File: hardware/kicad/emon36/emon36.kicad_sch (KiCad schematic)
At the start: 80 parts, among them J1 Barrel_Jack, J37 USB_B_Micro, J4 Barrel_Jack, SW1 SW_MEC_5E, SW2 SW_MEC_5E, SW3 SW_MEC_5E, SW4 SW_MEC_5E, SW5 RotaryEncoder, U1 ESP32-C3-WROOM-02-N4, U3 16.384MHz, U8 TPS5403

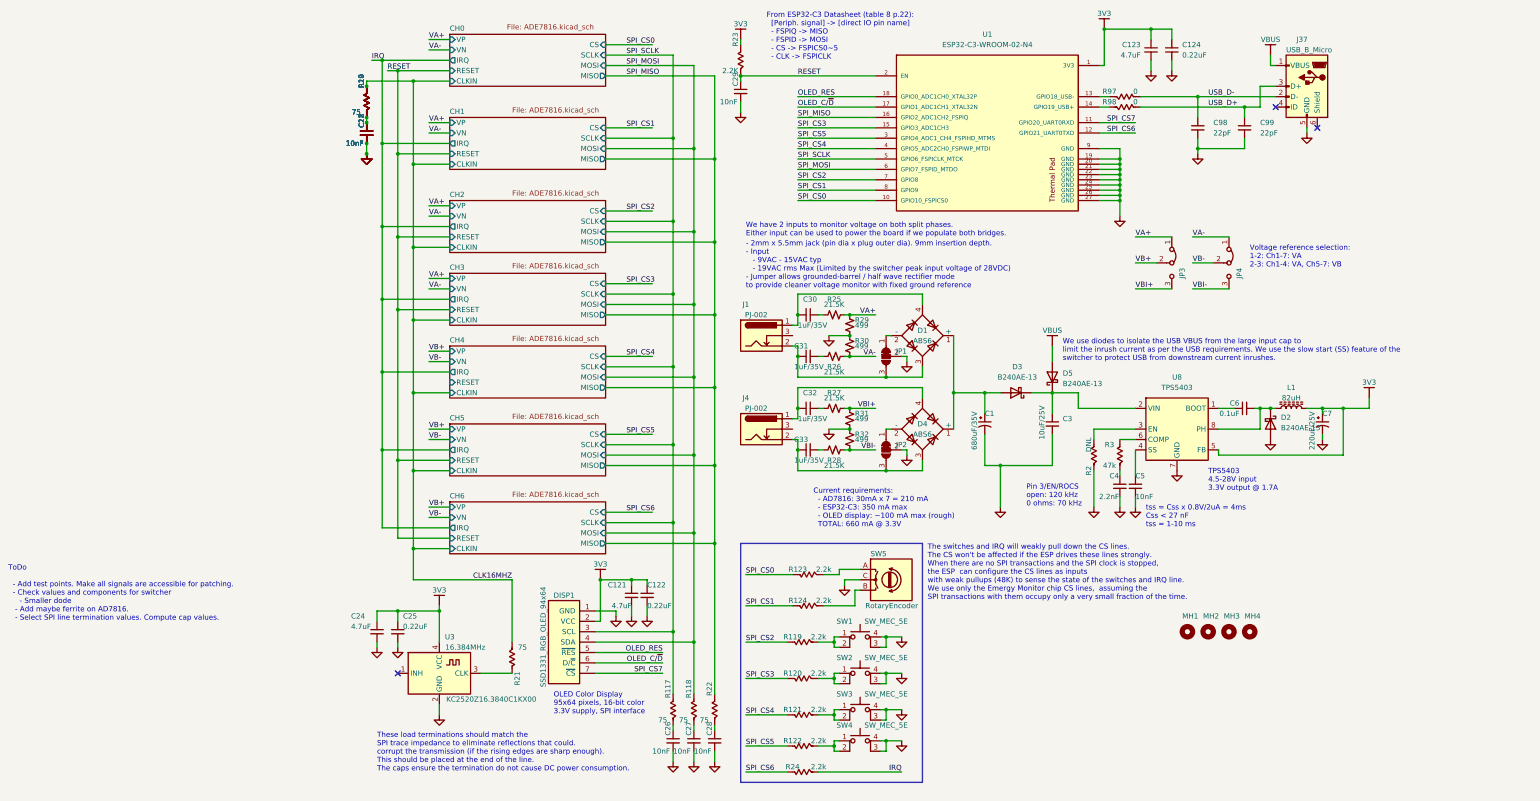
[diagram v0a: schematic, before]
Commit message: Finished schematics, layout and routing. Ready for verification.
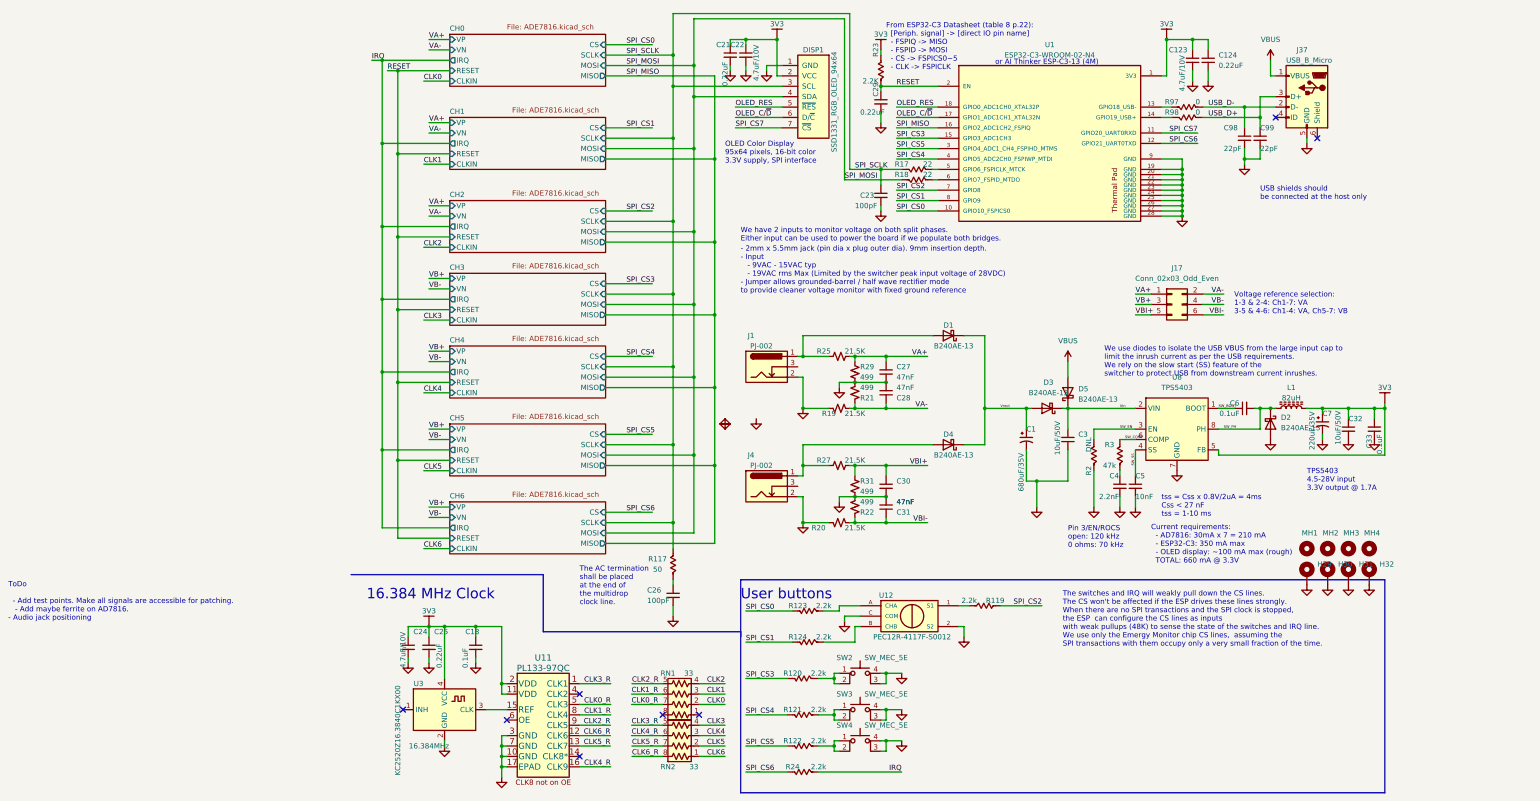
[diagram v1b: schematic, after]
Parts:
- removed C121: 4.7uF, Capacitor_SMD:C_0603_1608Metric, symbol Device:C_Small
- removed C122: 0.22uF, Capacitor_SMD:C_0603_1608Metric, symbol Device:C_Small
- removed D1, D4: ABS6, Diode_SMD:Diode_Bridge_Diotec_ABS, symbol Diode_Bridge:ABS6
- removed JP1, JP2: SolderJumper_3_Bridged12, Jumper:SolderJumper-3_P1.3mm_Bridged12_RoundedPad1.0x1.5mm, symbol Jumper:SolderJumper_3_Bridged12
- removed JP3, JP4: Jumper_3_Bridged12, Connector_PinHeader_2.54mm:PinHeader_1x03_P2.54mm_Vertical, symbol Jumper:Jumper_3_Bridged12
- removed R118, R19, R20, R21, R22: 75, Resistor_SMD:R_0603_1608Metric, symbol emon36:R_US
- removed R26, R28: 21.5K, Resistor_SMD:R_0603_1608Metric, symbol Device:R_Small_US
- removed R30, R32: 499, Resistor_SMD:R_0603_1608Metric, symbol Device:R_Small_US
- removed SW1: SW_MEC_5E, Button_Switch_SMD:SW_Push_1P1T_NO_6x6mm_H13mm, symbol Switch:SW_MEC_5E
- removed SW5: RotaryEncoder, Rotary_Encoder:RotaryEncoder_Alps_EC12E_Vertical_H20mm, symbol Device:RotaryEncoder
- added D1, D4: B240AE-13, Diode_SMD:D_SOD-123F, symbol Diode:B240
- added H29, H30, H31, H32: MountingHole_Pad, _Connector_Audio_local:STX-4335_Combined_Mounting_Hole, symbol Mechanical:MountingHole_Pad
- added J17: Conn_02x03_Odd_Even, Connector_PinHeader_2.54mm:PinHeader_2x03_P2.54mm_Vertical, symbol Connector_Generic:Conn_02x03_Odd_Even
- added R19, R20: 21.5K, Resistor_SMD:R_0603_1608Metric, symbol Device:R_Small_US
- added R21, R22: 499, Resistor_SMD:R_0603_1608Metric, symbol Device:R_Small_US
- added RN1, RN2: 33, _SnapEDA Library:RESCAV50P200X100X55-8N, symbol Device:R_Network04_US
- added U11: PL133-97QC, emon36:PL133-97QC, symbol PL133-97QC:PL133-97QC
- added U12: PEC12R-4117F-S0012, _SnapEDA Library:ENC_PEC12R-4025F-S0024, symbol PEC12R-4025F-S0024:PEC12R-4025F-S0024
- C1: footprint Capacitor_Tantalum_SMD:CP_EIA-1608-08_AVX-J -> Capacitor_THT:CP_Radial_D10.0mm_P5.00mm; MFR (none) -> Panasonic; MPN (none) -> EEU-FR1V681LB
- C123, C24: value 4.7uF -> 4.7uF/10V; Desc (none) -> CAP CER 4.7UF 10V X7S 0603; MFR (none) -> TDK Corporation; MPN (none) -> C1608X7S1A475K080AC
- C18: value 10nF -> 0.1uF
- C21, C29: value 10nF -> 0.22uF
- C22: value 10nF -> 4.7uF/10V; Desc (none) -> CAP CER 4.7UF 10V X7S 0603; MFR (none) -> TDK Corporation; MPN (none) -> C1608X7S1A475K080AC
- C23, C26: value 10nF -> 100pF
- C27, C28: value 10nF -> 47nF
- C3: value 10uF/25V -> 10uF/50V; footprint Capacitor_SMD:C_0603_1608Metric -> Capacitor_SMD:C_1206_3216Metric; Desc (none) -> CAP CER 10UF 50V X7R 1206; MFR (none) -> Samsung; MPN (none) -> CL31B106KBHNNNE
- C30, C31: value 1uF/35V -> 47nF
- C32: value 1uF/35V -> 10uF/50V; footprint Capacitor_SMD:C_0603_1608Metric -> Capacitor_SMD:C_1206_3216Metric; Desc (none) -> CAP CER 10UF 50V X7R 1206; MFR (none) -> Samsung; MPN (none) -> CL31B106KBHNNNE
- C33: value 1uF/35V -> 0.1uF
- C7: value 220uF/25V -> 220uF/35V; footprint Capacitor_Tantalum_SMD:CP_EIA-1608-08_AVX-J -> Capacitor_THT:CP_Radial_D10.0mm_P5.00mm; MFR (none) -> Robycon; MPN (none) -> 35YXF220MEFC10X12.5
- J4: footprint Connector_BarrelJack:BarrelJack_Horizontal -> emon36:PJ-002A
- R117: value 75 -> 50
- R17, R18: value 75 -> 22
- SW2, SW3, SW4: footprint Button_Switch_SMD:SW_Push_1P1T_NO_6x6mm_H13mm -> _Button_Switch_SMD:SW_Push_1P1T_NO_6x6mm_H13mm; symbol Switch:SW_MEC_5E -> emon36:SW_MEC_5E; MFR (none) -> C&K; MPN (none) -> PTS645SK13SMTR92LFS
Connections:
- net 3V3: now also C18.1, C21.1, C22.1, C32.1, C33.2, U11.11 (VDD), U11.2 (VDD); no longer D5.2 (A), J37.1 (VBUS)
- net GND: now also C30.2, C31.2, C32.2, C33.1, J1.2, J4.2, U1.28 (GND), U1.29 (GND), U1.30 (GND), U1.31 (GND), U1.32 (GND), U1.33 (GND), U1.34 (GND), U1.35 (GND), U1.36 (GND), U1.37 (GND), H29.1, H30.1, H31.1, H32.1, R19.1, R20.1, R21.2, R22.2, U11.10 (GND), U11.17 (EPAD), U11.3 (GND), U11.7 (GND), U12.2 (S2), U12.C (COM)
- net SPI_MOSI: now also R18.2; no longer U1.6 (GPIO7_FSPID_MTDO)
- net SPI_SCLK: now also C23.1, R17.2; no longer U1.5 (GPIO6_FSPICLK_MTCK)
- net VA+: now also C27.1, J17.1 (Pin_1)
- net VA-: now also C28.1, J17.2 (Pin_2), R19.2, R21.1
- net VB+: now also J17.3 (Pin_3)
- net VB-: now also J17.4 (Pin_4)
- net VBI+: now also C30.1, J17.5 (Pin_5)
- net VBI-: now also C31.1, J17.6 (Pin_6), R20.2, R22.1
- net Vin: now reaches C3.1, D3.1 (K), D5.1 (K), U8.2 (VIN)
- net at R25.1: now also J1.1, D1.2 (A); no longer C30.1
- net at R123.2: now also U12.A (CHA)
- net at R124.2: now also U12.B (CHB)
- net Vrect: now reaches C1.1, D3.2 (A)
- net Vrect: now also D1.1 (K), D4.1 (K)
- net at J4.1: now also R27.1, D4.2 (A); no longer C32.2
- net SW_BOOT: now reaches C6.1, U8.1 (BOOT)
- net SW_EN: now reaches R2.1, U8.3 (EN)
- net SW_SS: now reaches C5.1, U8.4 (SS)
- net SW_COMP: now reaches R3.1, U8.6 (COMP)
- net SW_PH: now reaches C6.2, D2.1 (K), L1.1, U8.8 (PH)
- net at U3.3 (CLK): now also U11.15 (REF)
- net at R119.2: now also U12.1 (S1)
- net CLK16MHZ: no longer names the net of R18.1
- net CLK16MHZ: now also U1.6 (GPIO7_FSPID_MTDO); no longer R17.1
- new net: R17.1, U1.5 (GPIO6_FSPICLK_MTCK)
- new net CLK0: RN1.2 (R2)
- new net CLK0_R: RN1.7 (R7), U11.5 (CLK3)
- new net CLK1: RN1.3 (R3)
- new net CLK1_R: RN1.6 (R6), U11.8 (CLK4)
- new net CLK2: RN1.4 (R4)
- new net CLK2_R: RN1.5 (R5), U11.9 (CLK5)
- new net CLK3: RN2.4 (R4)
- new net CLK3_R: RN2.5 (R5), U11.1 (CLK1)
- new net CLK4: RN2.3 (R3)
- new net CLK4_R: RN2.6 (R6), U11.16 (CLK9)
- new net CLK5: RN2.2 (R2)
- new net CLK5_R: RN2.7 (R7), U11.13 (CLK7)
- new net CLK6: RN2.1 (R1)
- new net CLK6_R: RN2.8 (R8), U11.12 (CLK6)
- new net VBUS: D5.2 (A), J37.1 (VBUS)
- no-connect marks 3 -> 8
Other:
- note added: "16.384 MHz Clock"
- note added: "The AC termination shall be placed at the end of the multidrop clock line."
- note added: "ToDo - Add test points. Make all signals are accessible for patching. - Add maybe ferrite on AD7816. - Audio jack positioning"
- note added: "USB shields should be connected at the host only"
- note added: "User buttons"
- note added: "Voltage reference selection: 1-3 & 2-4: Ch1-7: VA 3-5 & 4-6: Ch1-4: VA, Ch5-7: VB"
- note added: "We use diodes to isolate the USB VBUS from the large input cap to limit the inrush current as per the USB requirements. We rely on the slow start (SS) feature of the switcher to protect USB from downstream current inrushes."
- note added: "or AI Thinker ESP-C3-13 (4M)"
- note removed: "These load terminations should match the SPI trace impedance to eliminate reflections that could. corrupt the transmission (if the rising edges are sharp enough). This should be placed at the end of the line. The caps ensure the termination do not cause DC power consumption."
- note removed: "ToDo - Add test points. Make all signals are accessible for patching. - Check values and components for switcher - Smaller dode - Add maybe ferrite on AD7816. - Select SPI line termination values. Compute cap values."
- note removed: "Voltage reference selection: 1-2: Ch1-7: VA 2-3: Ch1-4: VA, Ch5-7: VB"
- note removed: "We use diodes to isolate the USB VBUS from the large input cap to limit the inrush current as per the USB requirements. We use the slow start (SS) feature of the switcher to protect USB from downstream current inrushes."
- moved on the sheet: C1, C123, C124, C24, C25, C26, C29, C3, C98, C99, D3, D5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
